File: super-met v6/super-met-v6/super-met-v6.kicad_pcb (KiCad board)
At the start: 2 copper layers, 99.3 x 99.3 mm, 57 parts, among them J1 Conn_01x02, J2 Conn_01x08, J3 Conn_01x08, J4 Conn_01x04, J5 Conn_01x08, J6 Conn_01x04, J7 Conn_01x02, J8 Conn_01x02, Q1 AO3400A, Q10 AO3400A, Q11 AO3400A, Q12 AO3400A, Q2 AO3400A, Q3 AO3400A, Q4 AO3400A, Q5 AO3400A, Q6 AO3400A, Q7 AO3400A, Q8 AO3400A, Q9 AO3400A, U1 DC-DC_MOD, U10 74HC595, U11 GY-GPS6MV2, U12 ESP-01v090, U13 74HC4052D, U14 BLUEPILL, U2 DC-DC_MOD, U3 DC-DC_MOD, U4 ADS1115IDGS, U5 ADS1115IDGS, U6 ADS1115IDGS, U7 ADS1115IDGS, U8 74HC595, U9 SIM800L

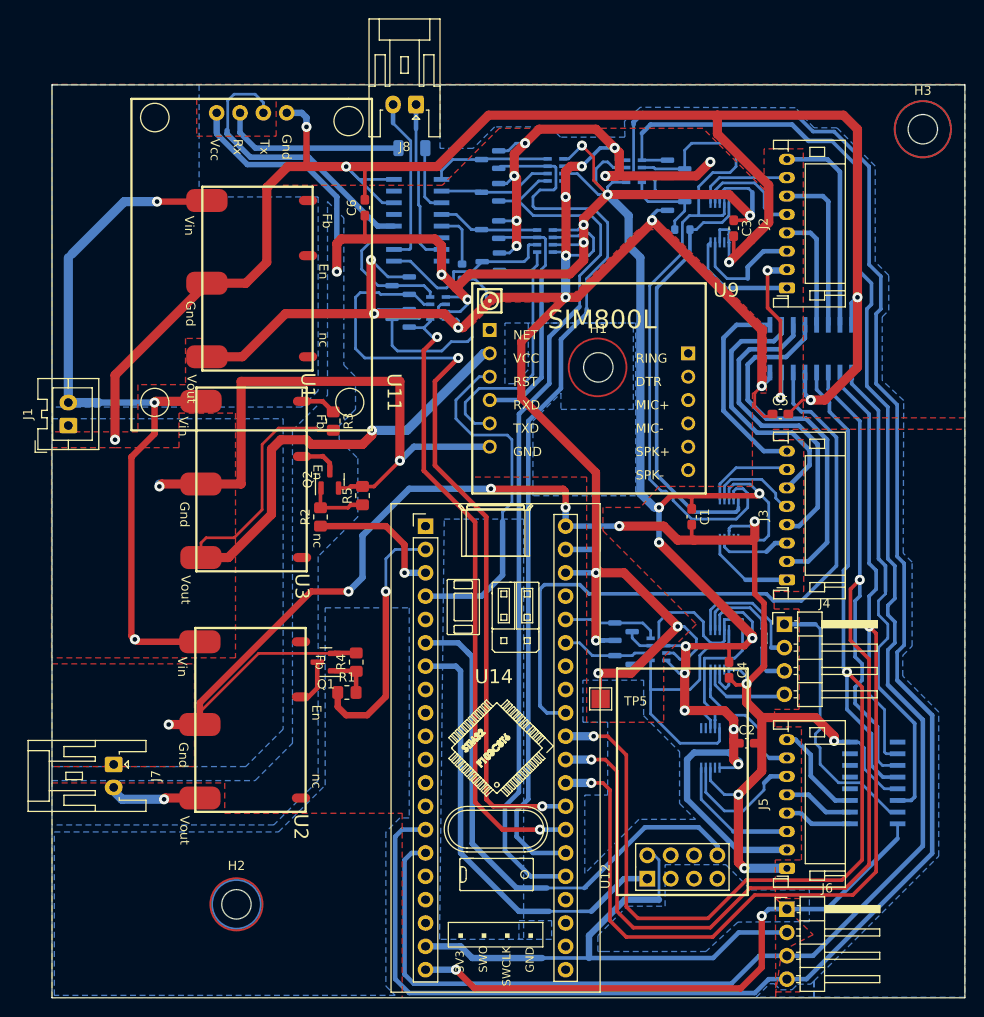
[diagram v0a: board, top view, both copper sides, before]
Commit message: preparing sensors board
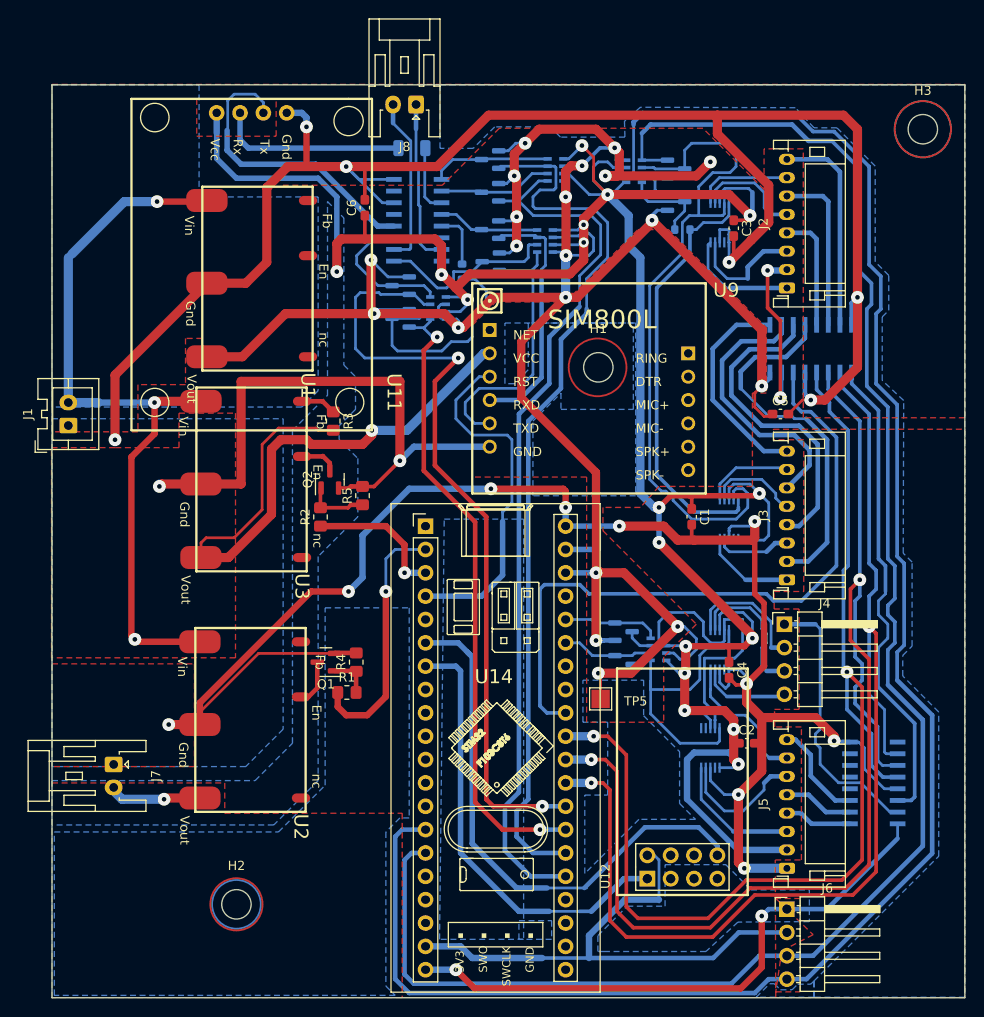
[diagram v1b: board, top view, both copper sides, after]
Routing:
- net 5.2v: track 301.8 -> 303.4 mm
- net /gps_tx: track 31.5 -> 32.6 mm
- net /s8_en_1: track 22.3 -> 23.3 mm
- net /s7_en_1: track 28.9 -> 29.7 mm
- net /s6_en_1: track 34.5 -> 35.1 mm

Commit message: 4 layer init
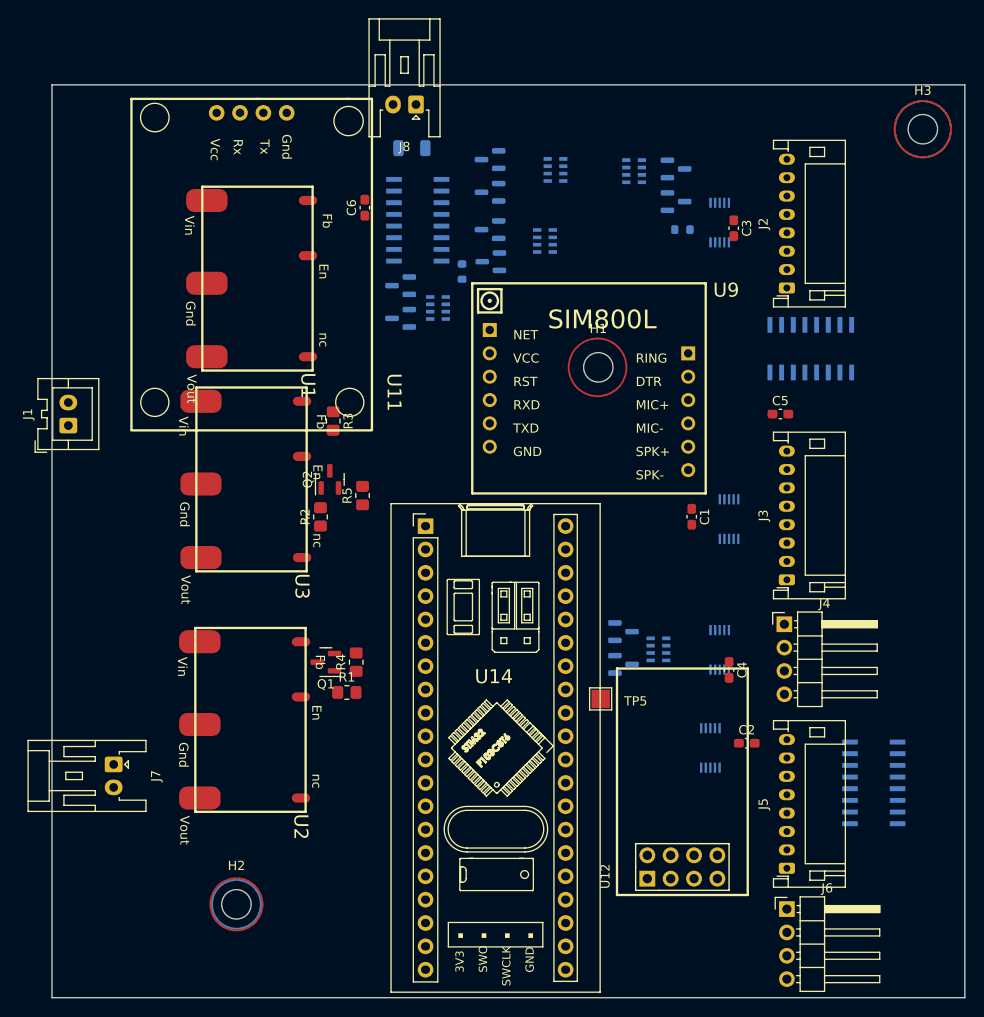
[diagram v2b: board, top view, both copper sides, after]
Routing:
- net GND: track 527.9 -> 0.00 mm, vias 18 -> 0
- net 3.3v: track 352.6 -> 0.00 mm, vias 22 -> 0
- net 5.2v: track 303.4 -> 0.00 mm, vias 18 -> 0
- net /SCL1: track 202.3 -> 0.00 mm
- net /SDA1: track 188.1 -> 0.00 mm
- net /sr_clk: track 132.5 -> 0.00 mm, vias 2 -> 0
- net /sr_clear: track 124.4 -> 0.00 mm, vias 2 -> 0
- net /sr_latch: track 122.9 -> 0.00 mm, vias 2 -> 0
- net /uart_mux_s1: track 98.4 -> 0.00 mm
- net /uart_mux_s0: track 96.4 -> 0.00 mm
- net /uart_mux_rx: track 86.6 -> 0.00 mm, vias 2 -> 0
- net /Power_Vin: track 85.8 -> 0.00 mm, vias 3 -> 0
- net Net-(Q4-Pad3): track 75.8 -> 0.00 mm
- net /sr_in: track 74.1 -> 0.00 mm
- net 4.2v: track 71.0 -> 0.00 mm, vias 1 -> 0
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- removed copper zone on B.Cu, net (none)
- removed copper zone on B.Cu, net /Power_Vin
- removed copper zone on F.Cu, net /Power_Vin
- removed copper zone on B.Cu, net 3.3v
- removed copper zone on F.Cu, net 3.3v
- removed copper zone on B.Cu, net 5.2v
- removed copper zone on F.Cu, net 5.2v
- removed copper zone on B.Cu, net GND
- removed copper zone on F.Cu, net GND
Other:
- copper layers 2 -> 4
